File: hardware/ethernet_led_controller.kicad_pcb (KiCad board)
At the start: 2 copper layers, 75.1 x 75 mm, 26 parts, among them J1 WeMos_CH340G_USB_to_SERIAL, J2 RJ45, J3 RJ45, J4 terminal_04, J5 terminal_04, J6 Barrel_Jack_Switch, J7 terminal_02, Q1 2N3904, Q2 2N3904, U1 WT32-ETH01, U2 74HC245

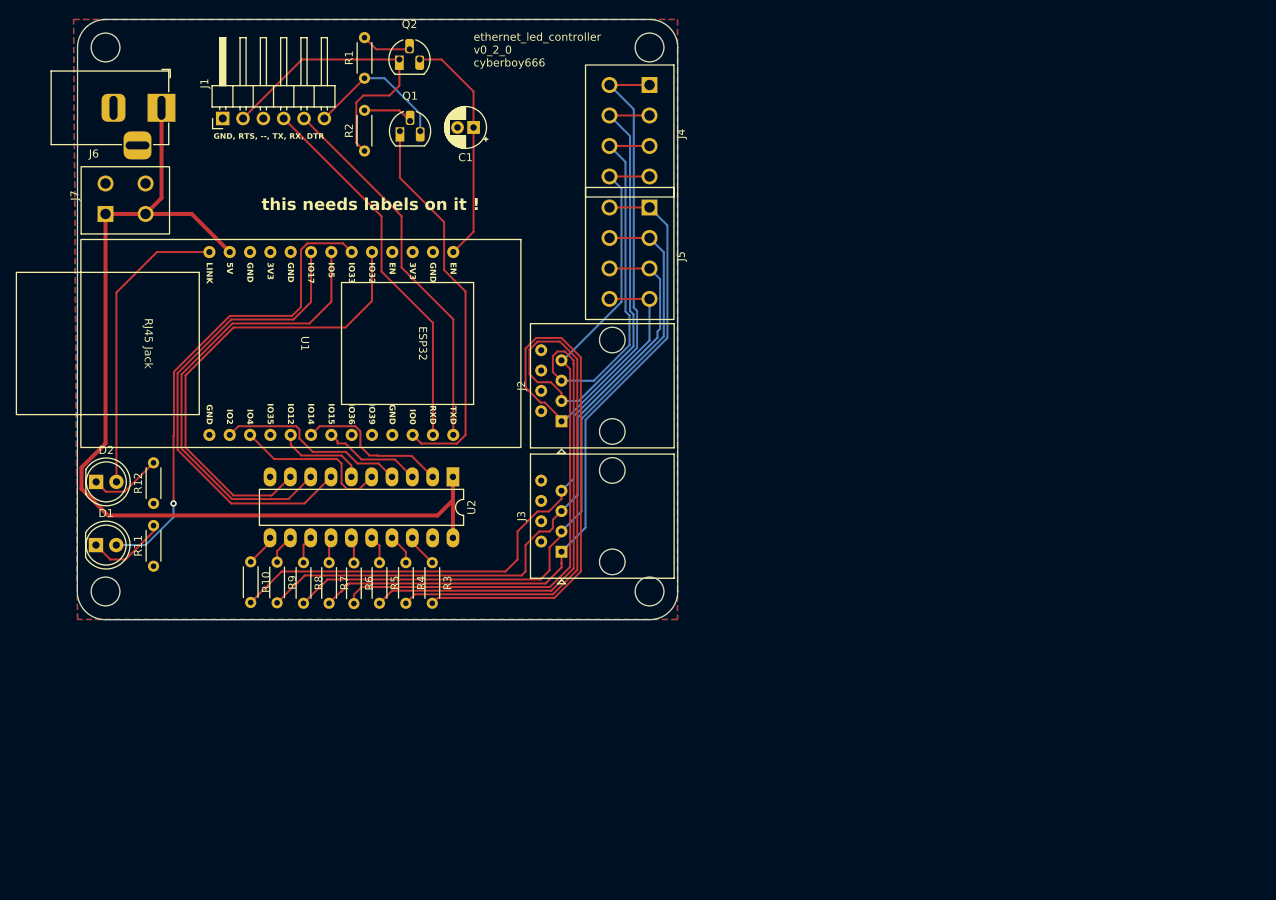
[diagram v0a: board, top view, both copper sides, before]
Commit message: update hardware and software
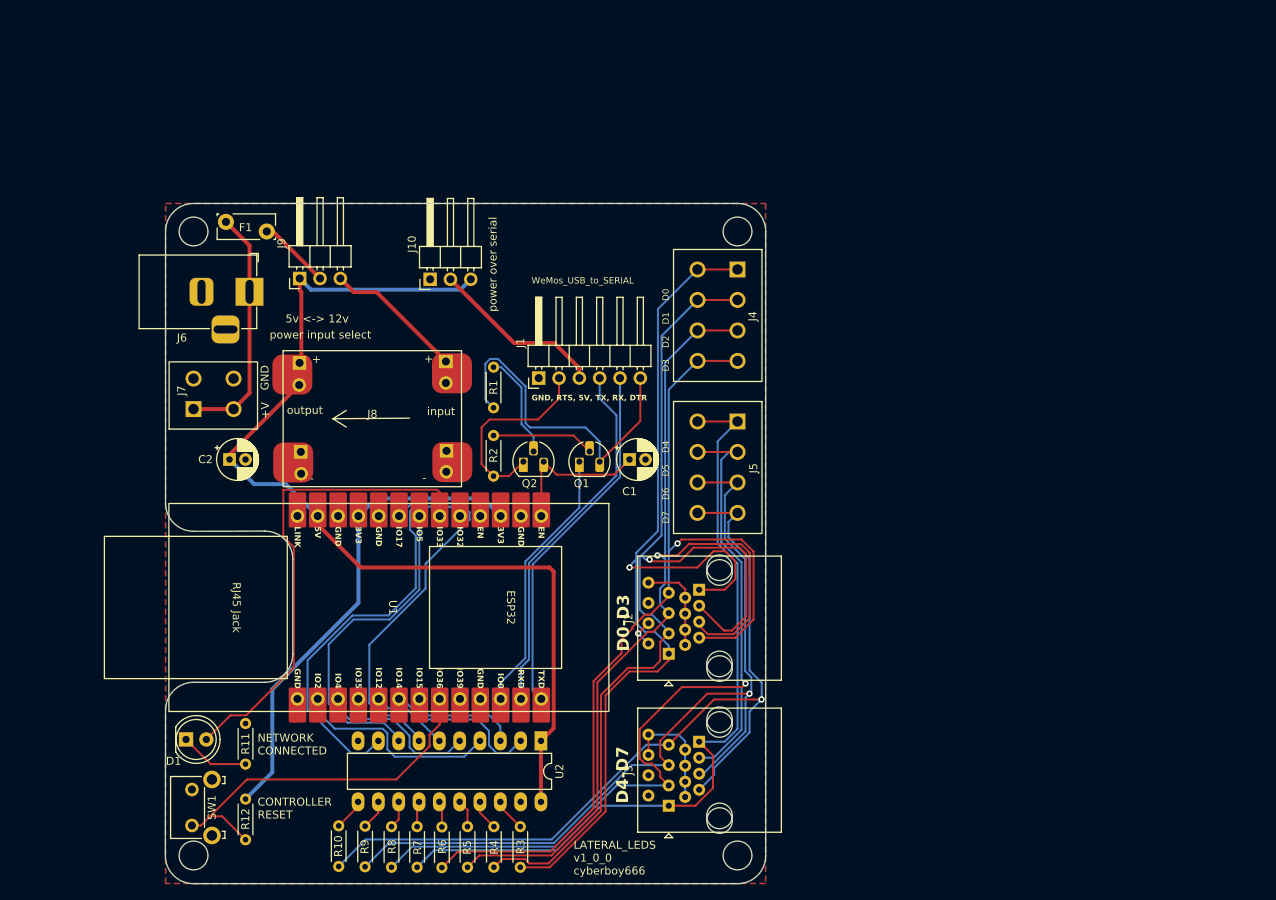
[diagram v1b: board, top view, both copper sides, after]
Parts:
- removed D2: LED, LED_THT:LED_D5.0mm
- added C2: 220u, Capacitor_THT:CP_Radial_D5.0mm_P2.00mm, F.Cu at (58.0, 82.0)
- added F1: Polyfuse, Fuse:Fuse_Bourns_MF-RG300, F.Cu at (57.5, 52.3)
- added J10: Conn_01x02, Connector_PinHeader_2.54mm:PinHeader_1x03_P2.54mm_Horizontal, F.Cu at (83.1, 59.5)
- added J8: MP1584EN_5v_stepdown, lib_fp:MP1584EN_stepdown_module, F.Cu at (75.8, 76.8)
- added J9: Conn_01x03, Connector_PinHeader_2.54mm:PinHeader_1x03_P2.54mm_Horizontal, F.Cu at (66.8, 59.4)
- added SW1: SW_Push, Button_Switch_THT:SW_Tactile_SKHH_Angled, F.Cu at (53.3, 127.8)
- C1: value C_Polarized_Small -> 10u
- J2, J3: footprint Connector_RJ:RJ45_Amphenol_54602-x08_Horizontal -> lib_fp:RJ45_Horizontal
- R12: value 100 -> 10k
- moved Q2 52.6 mm to (94.7, 82.3)
- moved J1 51.1 mm to (96.7, 71.8)
- moved Q1 47.0 mm to (101.7, 82.3)
- moved C1 45.9 mm to (108.0, 82.0), turned to 0 degrees
- moved R1 44.2 mm to (91.0, 75.5)
- moved R2 43.7 mm to (91.0, 84.1)
- moved R12 43.6 mm to (60.0, 129.5)
- moved R3 34.8 mm to (94.3, 127.9)
- moved R4 34.8 mm to (91.0, 127.9)
- moved R5 34.8 mm to (87.7, 127.9)
- moved R6 34.8 mm to (84.5, 127.9)
- moved R7 34.8 mm to (81.4, 127.9)
- moved R8 34.8 mm to (78.2, 127.9)
- moved U1 34.8 mm to (77.9, 100.5)
- moved U2 34.8 mm to (96.9, 117.2)
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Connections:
- J1 pad 3: unconnected-(J1-Pin_3-Pad3) -> Net-(J1-Pin_3)
- J6 pad 1: +5V -> Net-(J7-Pin_1)
- J6 pad 3: GND -> unconnected-(J6-Pad3)
- J7 pad 1: +5V -> Net-(J7-Pin_1)
- R12 pad 1: GND -> Net-(U1-IO36/ADC1_CH0/INPUT_ONLY)
- R12 pad 2: Net-(D2-K) -> +3V3
- U1 pad 10: unconnected-(U1-3.3V-Pad10) -> +3V3
- U1 pad 13: Net-(D2-A) -> unconnected-(U1-LINK_LED-Pad13)
- U1 pad 21: unconnected-(U1-IO36/ADC1_CH0/INPUT_ONLY-Pad21) -> Net-(U1-IO36/ADC1_CH0/INPUT_ONLY)
- U1 pad 3: unconnected-(U1-3.3V-Pad3) -> +3V3
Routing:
- net +3V3: track 0.00 -> 61.6 mm
- net Net-(U1-IO36/ADC1_CH0/INPUT_ONLY): track 0.00 -> 45.1 mm
- net Net-(D2-A): track 37.4 -> 0.00 mm
- net Net-(J7-Pin_1): track 0.00 -> 30.5 mm
- net GND: track 0.00 -> 29.9 mm, vias 0 -> 1
- net Net-(J4-Pin_4): track 87.7 -> 116.8 mm, vias 0 -> 1
- net Net-(J5-Pin_2): track 85.7 -> 112.9 mm, vias 0 -> 1
- net Net-(J5-Pin_4): track 80.8 -> 106.5 mm, vias 0 -> 1
- net Net-(J1-Pin_6): track 18.1 -> 42.5 mm
- net Net-(J5-Pin_3): track 83.9 -> 106.8 mm, vias 0 -> 1
- net Net-(J1-Pin_3): track 0.00 -> 22.0 mm
- net Net-(J4-Pin_3): track 100.2 -> 120.6 mm, vias 0 -> 1
- net Net-(J8-Pin_1): track 0.00 -> 17.5 mm
- net Net-(U1-IO5/BOOT_FLOAT): track 57.9 -> 41.7 mm
- net Net-(Q1-E): track 48.9 -> 33.7 mm
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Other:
- board size 75.1 x 75 mm -> 75.1 x 85 mm
- board text added: "+V"
- board text added: "5v <-> 12v"
- board text added: "CONTROLLER RESET"
- board text added: "D0-D3"
- board text added: "D3 D2 D1 D0"
- board text added: "D4-D7"
- board text added: "D7 D6 D5 D4"
- board text added: "GND"
- board text added: "GND, RTS, 5V, TX, RX, DTR"
- board text added: "LATERAL_LEDS v1_0_0 cyberboy666"
- board text added: "NETWORK CONNECTED"
- board text added: "WeMos_USB_to_SERIAL"
- board text added: "power input select"
- board text added: "power over serial"
- board text removed: "GND, RTS, --, TX, RX, DTR"
- board text removed: "ethernet_led_controller v0_2_0 cyberboy666"
- board text removed: "this needs labels on it !"

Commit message: updating hardware for v1_1_0 - change layouts etc
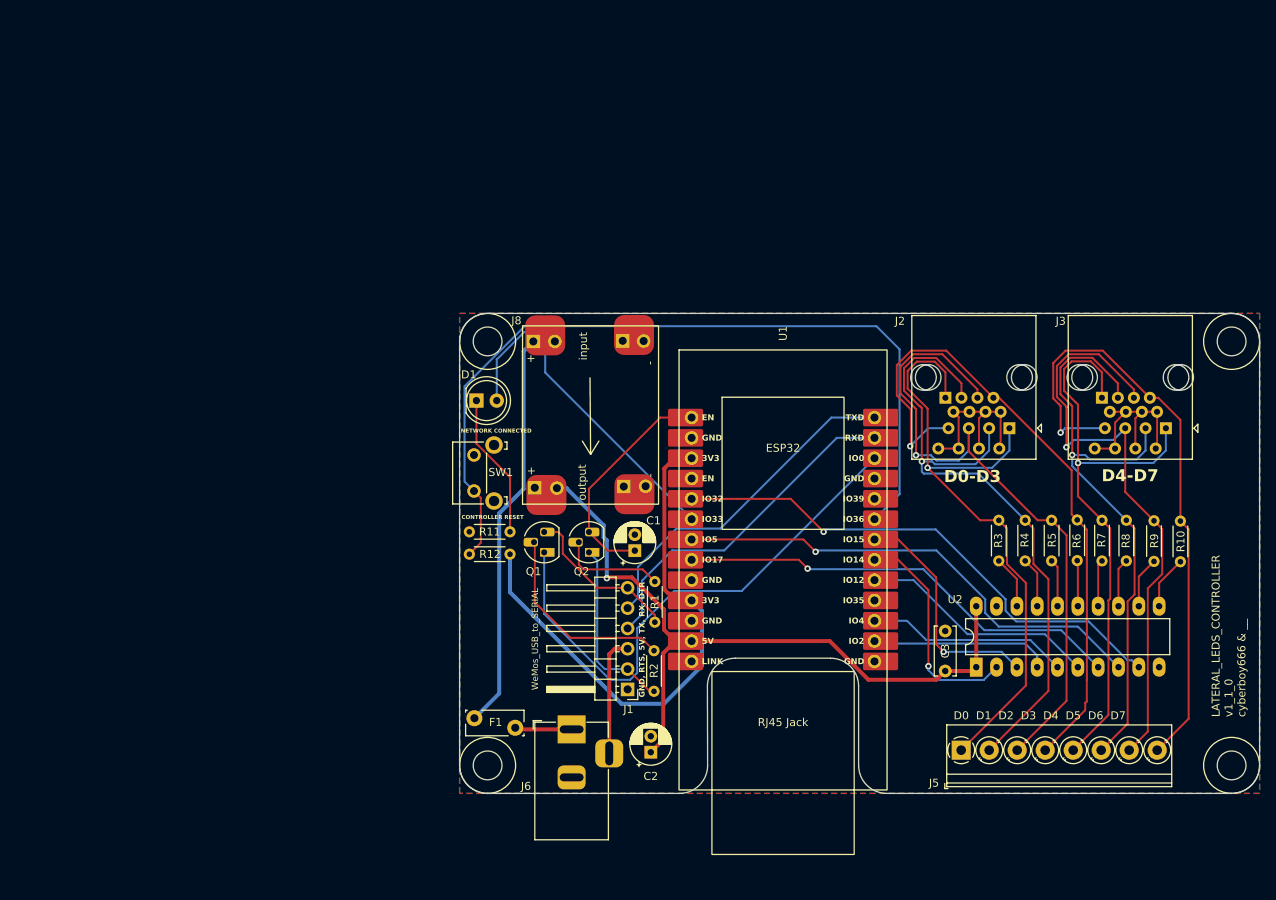
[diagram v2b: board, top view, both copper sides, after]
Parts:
- removed J10: Conn_01x02, Connector_PinHeader_2.54mm:PinHeader_1x03_P2.54mm_Horizontal
- removed J4: terminal_04, lib_fp:terminal_04
- removed J7: terminal_02, lib_fp:terminal_02
- removed J9: Conn_01x03, Connector_PinHeader_2.54mm:PinHeader_1x03_P2.54mm_Horizontal
- added C3: 0.1u, Capacitor_THT:C_Disc_D6.0mm_W2.5mm_P5.00mm, F.Cu at (147.5, 108.4)
- J5: value terminal_04 -> terminal_08; footprint lib_fp:terminal_04 -> TerminalBlock_Phoenix:TerminalBlock_Phoenix_PT-1,5-8-3.5-H_1x08_P3.50mm_Horizontal
- moved R10 110.3 mm to (176.9, 94.8), turned to 90 degrees
- moved R9 104.0 mm to (173.6, 94.7), turned to 90 degrees
- moved R8 97.7 mm to (170.1, 94.7), turned to 90 degrees
- moved R7 91.8 mm to (167.1, 94.7), turned to 90 degrees
- moved R6 86.1 mm to (164.0, 94.6), turned to 90 degrees
- moved R5 80.2 mm to (160.8, 94.7), turned to 90 degrees
- moved J3 78.0 mm to (175.0, 78.1), turned to 180 degrees
- moved R4 74.3 mm to (157.5, 94.7), turned to 90 degrees
- moved F1 72.8 mm to (93.7, 115.5), turned to 180 degrees
- moved R3 68.4 mm to (154.2, 94.7), turned to 90 degrees
- moved J6 67.9 mm to (100.8, 115.7), turned to 90 degrees
- moved C2 64.1 mm to (110.7, 118.6), turned to 90 degrees
- moved D1 55.8 mm to (88.9, 74.6)
- moved U2 55.2 mm to (151.3, 108.0), turned to 90 degrees
- moved SW1 54.7 mm to (88.6, 85.9)
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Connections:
- F1 pad 2: Net-(J9-Pin_2) -> Net-(J8-Pin_1)
- J2 pad 1: Net-(J4-Pin_1) -> Net-(J5-Pin_1)
- J2 pad 3: Net-(J4-Pin_2) -> Net-(J5-Pin_2)
- J2 pad 5: Net-(J4-Pin_3) -> Net-(J5-Pin_3)
- J2 pad 7: Net-(J4-Pin_4) -> Net-(J5-Pin_4)
- J3 pad 1: Net-(J5-Pin_1) -> Net-(J5-Pin_5)
- J3 pad 3: Net-(J5-Pin_2) -> Net-(J5-Pin_6)
- J3 pad 5: Net-(J5-Pin_3) -> Net-(J5-Pin_7)
- J3 pad 7: Net-(J5-Pin_4) -> Net-(J5-Pin_8)
- J6 pad 3: unconnected-(J6-Pad3) -> Net-(J1-Pin_3)
- R10 pad 2: Net-(J5-Pin_4) -> Net-(J5-Pin_8)
- R3 pad 2: Net-(J4-Pin_1) -> Net-(J5-Pin_1)
- R4 pad 2: Net-(J4-Pin_2) -> Net-(J5-Pin_2)
- R5 pad 2: Net-(J4-Pin_3) -> Net-(J5-Pin_3)
- R6 pad 2: Net-(J4-Pin_4) -> Net-(J5-Pin_4)
- R7 pad 2: Net-(J5-Pin_1) -> Net-(J5-Pin_5)
- R8 pad 2: Net-(J5-Pin_2) -> Net-(J5-Pin_6)
- R9 pad 2: Net-(J5-Pin_3) -> Net-(J5-Pin_7)
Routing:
- net Net-(J4-Pin_2): track 126.1 -> 0.00 mm, vias 1 -> 0
- net Net-(J4-Pin_3): track 120.6 -> 0.00 mm, vias 1 -> 0
- net Net-(J4-Pin_1): track 120.4 -> 0.00 mm, vias 1 -> 0
- net Net-(J4-Pin_4): track 116.8 -> 0.00 mm, vias 1 -> 0
- net Net-(J5-Pin_8): track 0.00 -> 78.3 mm, vias 0 -> 1
- net Net-(J5-Pin_6): track 0.00 -> 76.9 mm, vias 0 -> 1
- net Net-(J5-Pin_7): track 0.00 -> 76.0 mm, vias 0 -> 1
- net Net-(J5-Pin_5): track 0.00 -> 75.2 mm, vias 0 -> 1
- net Net-(U1-IO36/ADC1_CH0/INPUT_ONLY): track 45.1 -> 103.6 mm
- net Net-(Q1-E): track 33.7 -> 67.1 mm
- net Net-(J8-Pin_1): track 17.5 -> 50.1 mm
- net +5V: track 122.5 -> 92.3 mm, vias 0 -> 1
- net Net-(J5-Pin_2): track 112.9 -> 85.2 mm
- net Net-(F1-Pad1): track 30.5 -> 7.13 mm
- net Net-(J5-Pin_4): track 106.5 -> 83.4 mm
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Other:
- board size 75.1 x 85 mm -> 100 x 60 mm
- board text added: "D0 D1 D2 D3 D4 D5 D6 D7"
- board text added: "LATERAL_LEDS_CONTROLLER v1_1_0 cyberboy666 & __"
- board text removed: "+V"
- board text removed: "5v <-> 12v"
- board text removed: "D3 D2 D1 D0"
- board text removed: "D7 D6 D5 D4"
- board text removed: "GND"
- board text removed: "LATERAL_LEDS v1_0_0 cyberboy666"
- board text removed: "power input select"
- board text removed: "power over serial"
